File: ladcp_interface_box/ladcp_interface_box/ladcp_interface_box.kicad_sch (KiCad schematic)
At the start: 2 parts, among them J1 TERM BLK 8POS SIDE ENTRY 5MM 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, U1 FT4232H

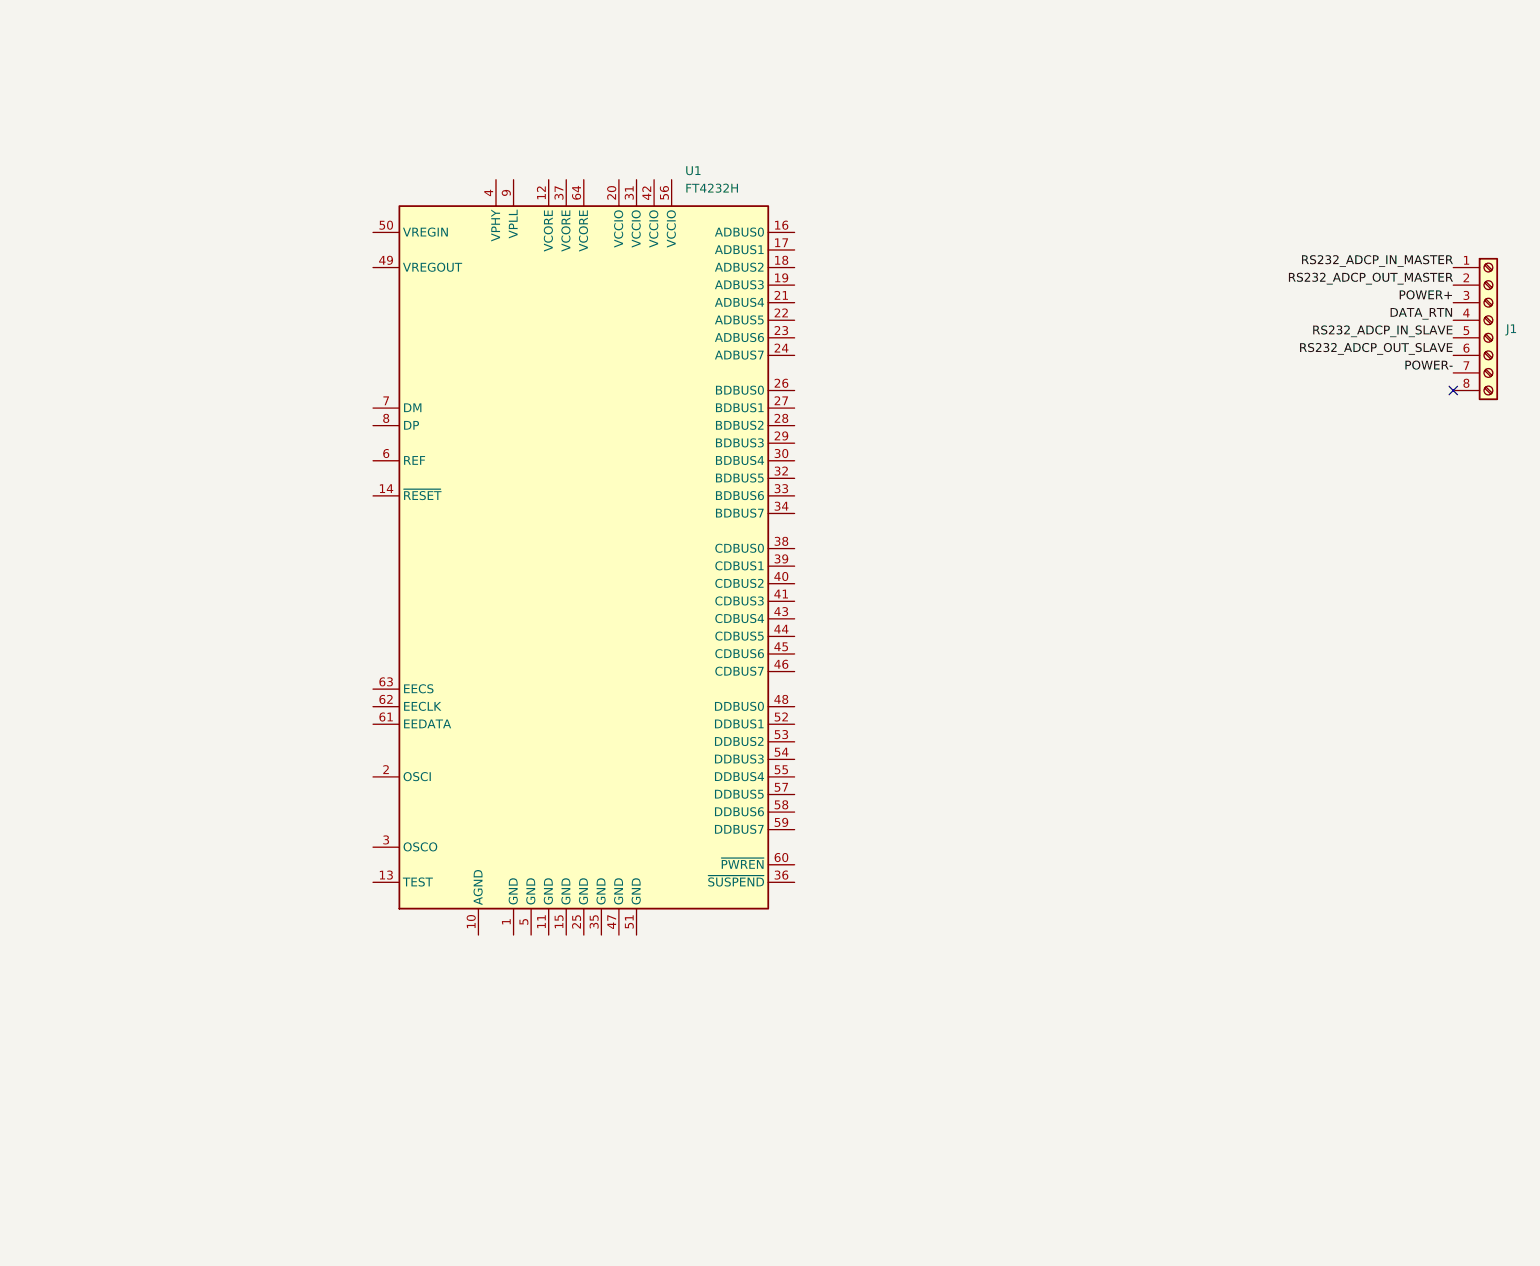
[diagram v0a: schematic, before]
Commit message: updated files
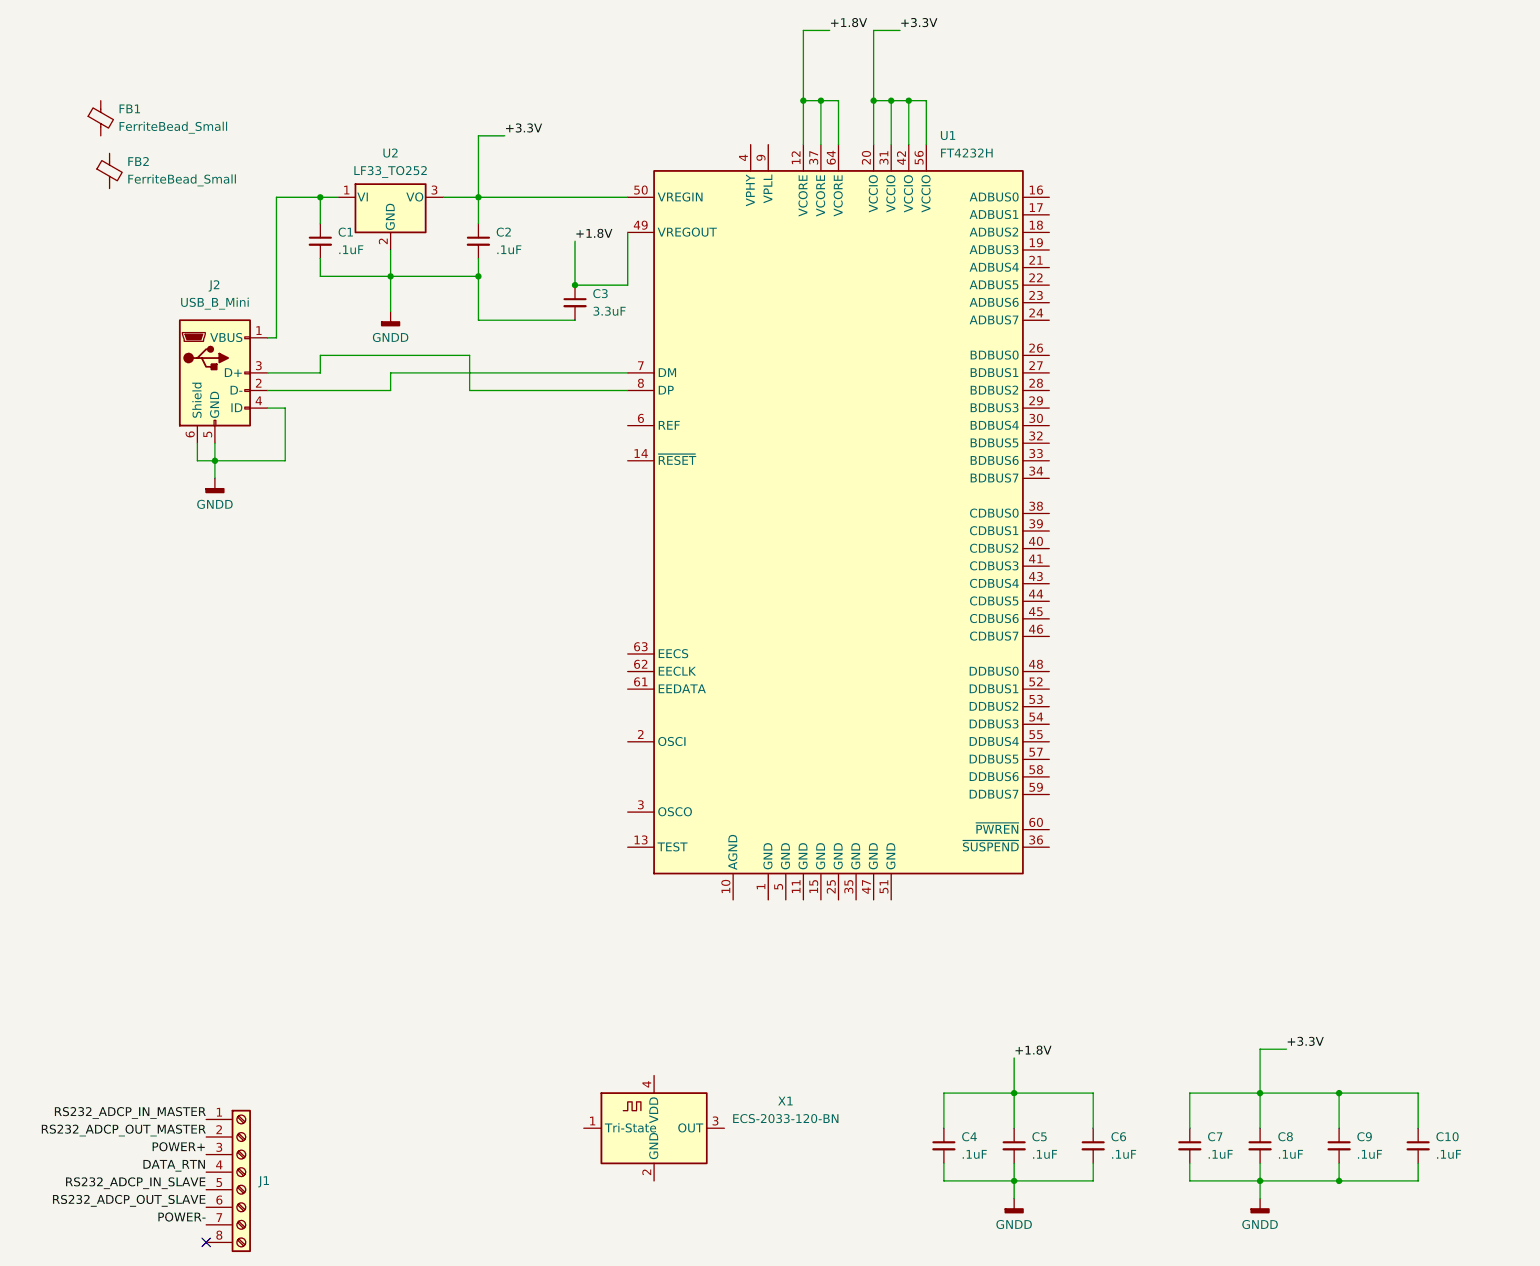
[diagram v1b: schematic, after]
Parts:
- added C1, C10, C2, C4, C5, C6, C7, C8, C9: .1uF, Capacitor_SMD:C_0805_2012Metric_Pad1.18x1.45mm_HandSolder, symbol Device:C_Small
- added C3: 3.3uF, Capacitor_SMD:C_0805_2012Metric_Pad1.18x1.45mm_HandSolder, symbol Device:C_Small
- added FB1, FB2: FerriteBead_Small, Inductor_SMD:L_0805_2012Metric_Pad1.15x1.40mm_HandSolder, symbol Device:FerriteBead_Small
- added J2: USB_B_Mini, Connector_USB:USB_Mini-B_Wuerth_65100516121_Horizontal, symbol Connector:USB_B_Mini
- added U2: LF33_TO252, Package_TO_SOT_SMD:TO-252-3_TabPin2, symbol Regulator_Linear:LF33_TO252
- added X1: ECS-2033-120-BN, Oscillator:Oscillator_SMD_ECS_2520MV-xxx-xx-4Pin_2.5x2.0mm, symbol Oscillator:ECS-2520MV-xxx-xx
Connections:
- net +1.8V: now reaches U1.12 (VCORE)
- net +1.8V: now also U1.37 (VCORE), U1.49 (VREGOUT), U1.64 (VCORE), C3.1, C4.1, C5.1, C6.1
- net +3.3V: now reaches U1.20 (VCCIO)
- net +3.3V: now also U1.31 (VCCIO), U1.42 (VCCIO), U1.50 (VREGIN), U1.56 (VCCIO), C10.1, C2.1, C7.1, C8.1, C9.1, U2.3 (VO)
- net at U1.7 (DM): now also J2.2 (D-)
- net at U1.8 (DP): now also J2.3 (D+)
- new net: C1.1, J2.1 (VBUS), U2.1 (VI)
- new net GNDD: C1.2, C10.2, C2.2, C3.2, C4.2, C5.2, C6.2, C7.2, C8.2, C9.2, J2.4 (ID), J2.5 (GND), J2.6 (Shield), U2.2 (GND)
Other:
- moved on the sheet: J1, U1
